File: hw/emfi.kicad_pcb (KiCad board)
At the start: 2 copper layers, 132.5 x 38 mm, 81 parts, among them J1 USB_B_Micro, J2 Conn_Coaxial, J3 Conn_Coaxial, J4 Conn_01x02, J5 Conn_01x03, J6 Conn_Coaxial, Q1 STT6N3LLH6, Q2 IKW40N120H3FKSA1, U1 STM32F205RETx, U2 FT232RL, U3 MIC2288, U4 LD1117S33TR_SOT223, U5 LD1117S33TR_SOT223, U6 MCP1407-E/SN, U7 SCS-200LD, U8 74LVC1G32

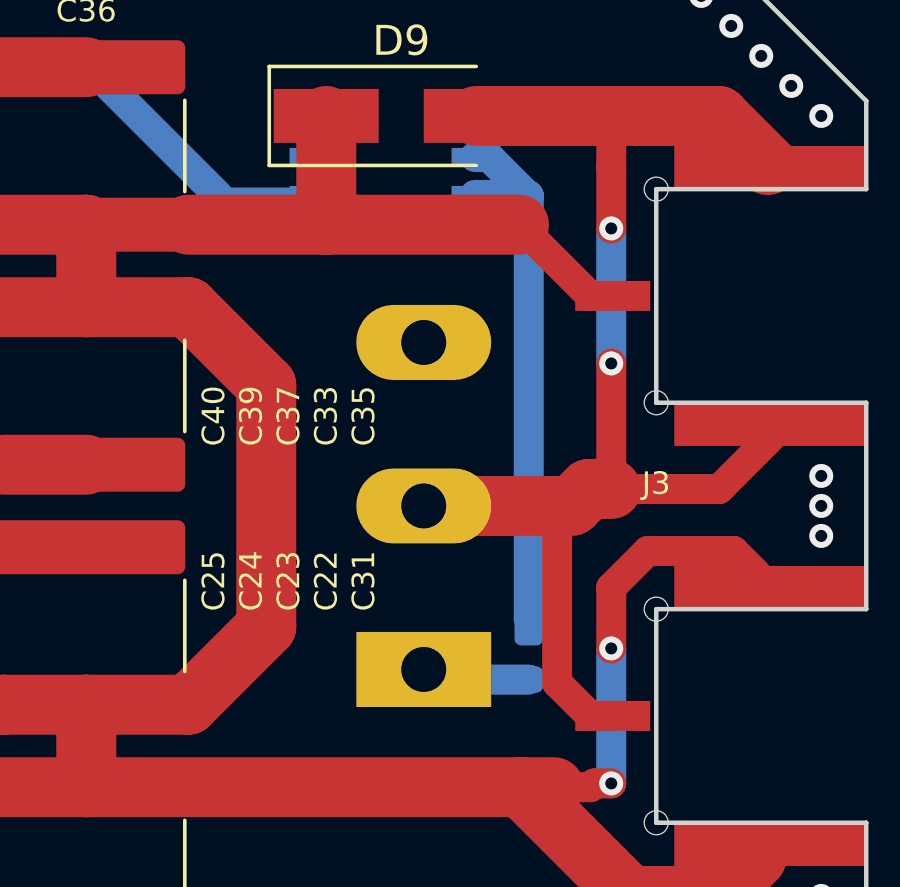
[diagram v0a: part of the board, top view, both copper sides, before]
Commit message: Fixed IGBT footprint.
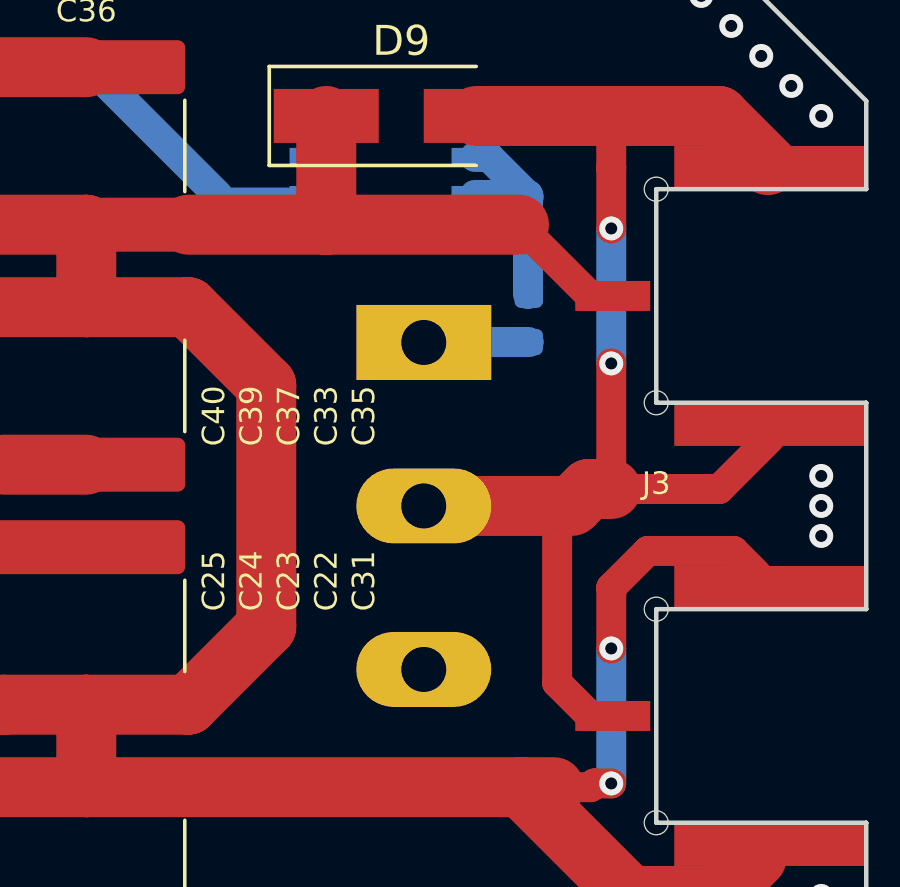
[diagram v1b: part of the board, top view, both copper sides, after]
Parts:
- Q2: footprint mykicadlibs:TO-247-3_Horizontal_TabUp_NoTabDrill -> mykicadlibs:TO-247-3_Horizontal_TabDown_NoTabDrill
- moved R9 11.2 mm to (164.2, 40.8)
- moved Q2 10.9 mm to (160.8, 41.5), turned to 270 degrees
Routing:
- net Net-(R9-Pad2): track 18.3 -> 7.43 mm
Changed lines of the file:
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@@
     (thickness 1.6)
     (drawings 32)
-    (tracks 720)
+    (tracks 719)
     (zones 0)
     (modules 81)
@@
     (uvia_dia 0.3)
     (uvia_drill 0.1)
-    (add_net /mcu/SW_SHOOT)
     (add_net GND)
     (add_net "Net-(J2-Pad1)")
@@
     (add_net "Net-(C20-Pad1)")
     (add_net "Net-(C21-Pad1)")
-    (add_net "Net-(Q2-Pad1)")
   )
   (net_class "Low Voltage" ""
@@
     (add_net /mcu/ADC)
     (add_net /mcu/RX)
+    (add_net /mcu/SW_SHOOT)
     (add_net "Net-(C6-Pad1)")
     (add_net "Net-(C7-Pad1)")
@@
     (add_net "Net-(J5-Pad2)")
     (add_net "Net-(Q1-Pad1)")
+    (add_net "Net-(Q2-Pad1)")
     (add_net "Net-(R10-Pad2)")
     (add_net "Net-(R5-Pad2)")
@@
     (add_net "Net-(U6-Pad3)")
   )
+  (module mykicadlibs:TO-247-3_Horizontal_TabDown_NoTabDrill (layer B.Cu)
+    (at 160.75 41.55 270)
+    (descr "TO-247-3, Horizontal, RM 5.45mm, see https://toshiba.semicon-storage.com/us/product/mosfet/to-247-4l.html")
+    (tags "TO-247-3 Horizontal RM 5.45mm")
+    (fp_text reference Q2 (at 5.45 27.15 270) (layer B.SilkS)
+      (effects (font (size 1 1) (thickness 0.15)) (justify mirror))
+    )
+    (fp_text value IKW40N120H3FKSA1 (at 5.45 -3.25 270) (layer B.Fab)
+      (effects (font (size 1 1) (thickness 0.15)) (justify mirror))
+    )
+    (fp_circle (center 5.45 19.86) (end 7.255 19.86) (layer B.Fab) (width 0.1))
+    (fp_line (start -2.5 5.08) (end -2.5 26.03) (layer B.Fab) (width 0.1))
+    (fp_line (start -2.5 26.03) (end 13.4 26.03) (layer B.Fab) (width 0.1))
+    (fp_line (start 13.4 26.03) (end 13.4 5.08) (layer B.Fab) (width 0.1))
+    (fp_line (start 13.4 5.08) (end -2.5 5.08) (layer B.Fab) (width 0.1))
+    (fp_line (start 0 5.08) (end 0 0) (layer B.Fab) (width 0.1))
+    (fp_line (start 5.45 5.08) (end 5.45 0) (layer B.Fab) (width 0.1))
+    (fp_line (start 10.9 5.08) (end 10.9 0) (layer B.Fab) (width 0.1))
+    (fp_line (start -2.62 4.96) (end 13.52 4.96) (layer B.SilkS) (width 0.12))
+    (fp_line (start -2.62 26.15) (end 13.52 26.15) (layer B.SilkS) (width 0.12))
+    (fp_line (start -2.62 26.15) (end -2.62 4.96) (layer B.SilkS) (width 0.12))
+    (fp_line (start 13.52 26.15) (end 13.52 4.96) (layer B.SilkS) (width 0.12))
+    (fp_line (start 0 4.96) (end 0 2.4) (layer B.SilkS) (width 0.12))
+    (fp_line (start 5.45 4.96) (end 5.45 2.4) (layer B.SilkS) (width 0.12))
+    (fp_line (start 10.9 4.96) (end 10.9 2.4) (layer B.SilkS) (width 0.12))
+    (fp_line (start -2.75 26.28) (end -2.75 -2.5) (layer B.CrtYd) (width 0.05))
+    (fp_line (start -2.75 -2.5) (end 13.65 -2.5) (layer B.CrtYd) (width 0.05))
+    (fp_line (start 13.65 -2.5) (end 13.65 26.28) (layer B.CrtYd) (width 0.05))
+    (fp_line (start 13.65 26.28) (end -2.75 26.28) (layer B.CrtYd) (width 0.05))
+    (fp_text user %R (at 5.45 27.15 270) (layer B.Fab)
+      (effects (font (size 1 1) (thickness 0.15)) (justify mirror))
+    )
+    (pad 1 thru_hole rect (at 0 0 270) (size 2.5 4.5) (drill 1.5) (layers *.Cu *.Mask)
+      (net 7 "Net-(Q2-Pad1)"))
+    (pad 2 thru_hole oval (at 5.45 0 270) (size 2.5 4.5) (drill 1.5) (layers *.Cu *.Mask)
+      (net 8 /analog/ANTENNA_B))
+    (pad 3 thru_hole oval (at 10.9 0 270) (size 2.5 4.5) (drill 1.5) (layers *.Cu *.Mask)
+      (net 1 GND))
+    (model /home/ohe/projects/mykicadlibs/3d/to-247-3-bend.wrl
+      (at (xyz 0 0 0))
+      (scale (xyz 1 1 1))
+      (rotate (xyz 0 0 90))
+    )
+  )
   (module Resistor_SMD:R_0603_1608Metric (layer B.Cu)
     (at 71 39.5 270)
@@
   )
   (module Resistor_SMD:R_0603_1608Metric (layer B.Cu)
-    (at 164.25 52 90)
+    (at 164.25 40.75 90)
     (descr "Resistor SMD 0603 (1608 Metric), square (rectangular) end terminal, IPC_7351 nominal, (Body size source: http://www.tortai-tech.com/upload/download/2011102023233369053.pdf), generated with kicad-footprint-generator")
     (tags resistor)
@@
     )
   )
-  (module mykicadlibs:TO-247-3_Horizontal_TabUp_NoTabDrill (layer B.Cu)
-    (at 160.75 52.45 90)
-    (descr "TO-247-3, Horizontal, RM 5.45mm, see https://toshiba.semicon-storage.com/us/product/mosfet/to-247-4l.html")
-    (tags "TO-247-3 Horizontal RM 5.45mm")
-    (fp_text reference Q2 (at 5.45 -27.15 180) (layer B.SilkS)
-      (effects (font (size 0.75 0.75) (thickness 0.125)) (justify mirror))
-    )
-    (fp_text value IKW40N120H3FKSA1 (at 5.45 3.25 90) (layer B.Fab)
-      (effects (font (size 1 1) (thickness 0.15)) (justify mirror))
-    )
-    (fp_circle (center 5.45 -19.86) (end 7.255 -19.86) (layer B.Fab) (width 0.1))
-    (fp_line (start -2.5 -5.08) (end -2.5 -26.03) (layer B.Fab) (width 0.1))
-    (fp_line (start -2.5 -26.03) (end 13.4 -26.03) (layer B.Fab) (width 0.1))
-    (fp_line (start 13.4 -26.03) (end 13.4 -5.08) (layer B.Fab) (width 0.1))
-    (fp_line (start 13.4 -5.08) (end -2.5 -5.08) (layer B.Fab) (width 0.1))
-    (fp_line (start 0 -5.08) (end 0 0) (layer B.Fab) (width 0.1))
-    (fp_line (start 5.45 -5.08) (end 5.45 0) (layer B.Fab) (width 0.1))
-    (fp_line (start 10.9 -5.08) (end 10.9 0) (layer B.Fab) (width 0.1))
-    (fp_line (start -2.62 -4.96) (end 13.52 -4.96) (layer B.SilkS) (width 0.12))
-    (fp_line (start -2.62 -26.15) (end 13.52 -26.15) (layer B.SilkS) (width 0.12))
-    (fp_line (start -2.62 -4.96) (end -2.62 -26.15) (layer B.SilkS) (width 0.12))
-    (fp_line (start 13.52 -4.96) (end 13.52 -26.15) (layer B.SilkS) (width 0.12))
-    (fp_line (start 0 -2.4) (end 0 -4.96) (layer B.SilkS) (width 0.12))
-    (fp_line (start 5.45 -2.4) (end 5.45 -4.96) (layer B.SilkS) (width 0.12))
-    (fp_line (start 10.9 -2.4) (end 10.9 -4.96) (layer B.SilkS) (width 0.12))
-    (fp_line (start -2.75 2.5) (end -2.75 -26.28) (layer B.CrtYd) (width 0.05))
-    (fp_line (start -2.75 -26.28) (end 13.65 -26.28) (layer B.CrtYd) (width 0.05))
-    (fp_line (start 13.65 -26.28) (end 13.65 2.5) (layer B.CrtYd) (width 0.05))
-    (fp_line (start 13.65 2.5) (end -2.75 2.5) (layer B.CrtYd) (width 0.05))
-    (fp_text user %R (at 5.45 -27.15 90) (layer B.Fab)
-      (effects (font (size 1 1) (thickness 0.15)) (justify mirror))
-    )
-    (pad 1 thru_hole rect (at 0 0 90) (size 2.5 4.5) (drill 1.5) (layers *.Cu *.Mask)
-      (net 7 "Net-(Q2-Pad1)"))
-    (pad 2 thru_hole oval (at 5.45 0 90) (size 2.5 4.5) (drill 1.5) (layers *.Cu *.Mask)
-      (net 8 /analog/ANTENNA_B))
-    (pad 3 thru_hole oval (at 10.9 0 90) (size 2.5 4.5) (drill 1.5) (layers *.Cu *.Mask)
-      (net 1 GND))
-    (model /home/ohe/projects/mykicadlibs/3d/to-247-3-bend.wrl
-      (offset (xyz 10.9 0 0))
-      (scale (xyz 1 1 1))
-      (rotate (xyz 0 0 -90))
-    )
-  )
   (module mykicadlibs:SCS-200L (layer F.Cu)
     (at 87.63 47.49 180)
@@
   (segment (start 56.55 54.7) (end 55.25 56) (width 0.25) (layer F.Cu) (net 6))
   (segment (start 58.2 54.7) (end 56.55 54.7) (width 0.25) (layer F.Cu) (net 6))
-  (segment (start 161.0875 52.7875) (end 160.75 52.45) (width 1) (layer B.Cu) (net 7))
-  (segment (start 164.25 52.7875) (end 161.0875 52.7875) (width 1) (layer B.Cu) (net 7))
+  (segment (start 161.0875 52.7875) (end 160.75 52.45) (width 1) (layer B.Cu) (net 1))
+  (segment (start 160.7625 41.5375) (end 160.75 41.55) (width 1) (layer B.Cu) (net 7))
+  (segment (start 164.25 41.5375) (end 160.7625 41.5375) (width 1) (layer B.Cu) (net 7))
   (segment (start 170.60001 46.435) (end 172.3 44.73501) (width 1) (layer F.Cu) (net 8))
   (via (at 167 42.25) (size 0.8) (drill 0.4) (layers F.Cu B.Cu) (net 8))
@@
   (segment (start 87.63 42.37) (end 90.96 39.04) (width 1) (layer F.Cu) (net 85))
   (segment (start 87.63 45.685) (end 87.63 42.37) (width 1) (layer F.Cu) (net 85))
-  (segment (start 164.25 36.69) (end 164.25 50.8) (width 1) (layer B.Cu) (net 86))
   (segment (start 162.925 35.365) (end 162.45 35.365) (width 1) (layer B.Cu) (net 86))
   (segment (start 164.25 36.69) (end 162.925 35.365) (width 1) (layer B.Cu) (net 86))
-  (segment (start 164.25 36.66) (end 164.25 36.69) (width 1) (layer B.Cu) (net 86))
-  (segment (start 164.225 36.635) (end 164.25 36.66) (width 1) (layer B.Cu) (net 86))
   (segment (start 162.45 36.635) (end 164.225 36.635) (width 1) (layer B.Cu) (net 86))
+  (segment (start 164.225 36.635) (end 164.225 39.93749) (width 1) (layer B.Cu) (net 86))
   (via (at 63.95 57.5) (size 0.8) (drill 0.4) (layers F.Cu B.Cu) (net 88))
   (segment (start 63.65 58.65) (end 63.65 57.8) (width 0.25) (layer F.Cu) (net 88))

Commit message: Upgraded files for KiCad 6
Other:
- net class Default removed
- net class High Voltage removed
- net class Low Voltage removed
